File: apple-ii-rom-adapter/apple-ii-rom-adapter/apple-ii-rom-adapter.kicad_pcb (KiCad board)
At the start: 2 copper layers, 51.6 x 43.9 mm, 11 parts, among them J1 ROMSEL, J2 9316 insert, J3 74LS138 insert, U1 28C256, U2 74LS00, U3 74LS138

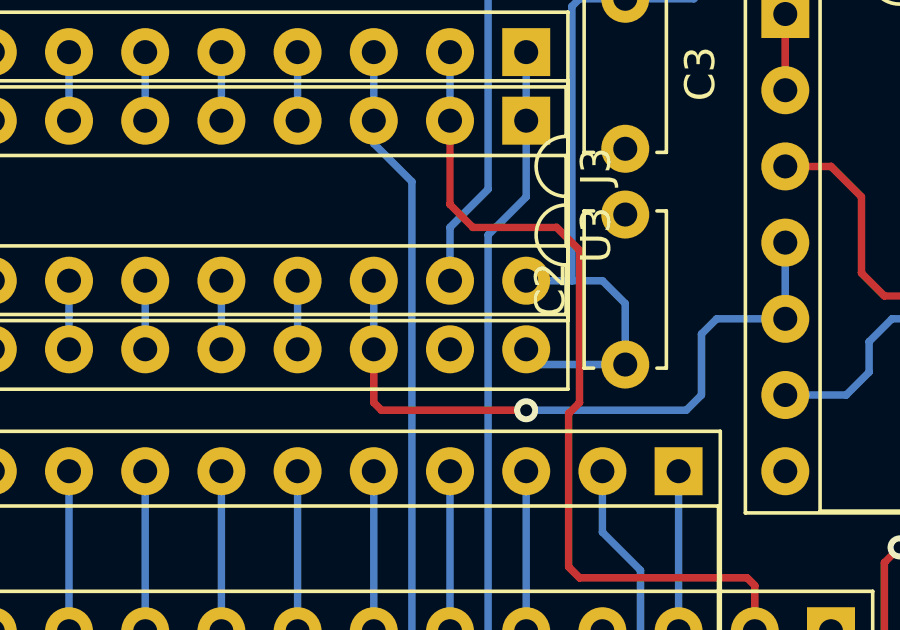
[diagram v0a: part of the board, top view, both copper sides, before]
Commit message: whoops, missed a connection!
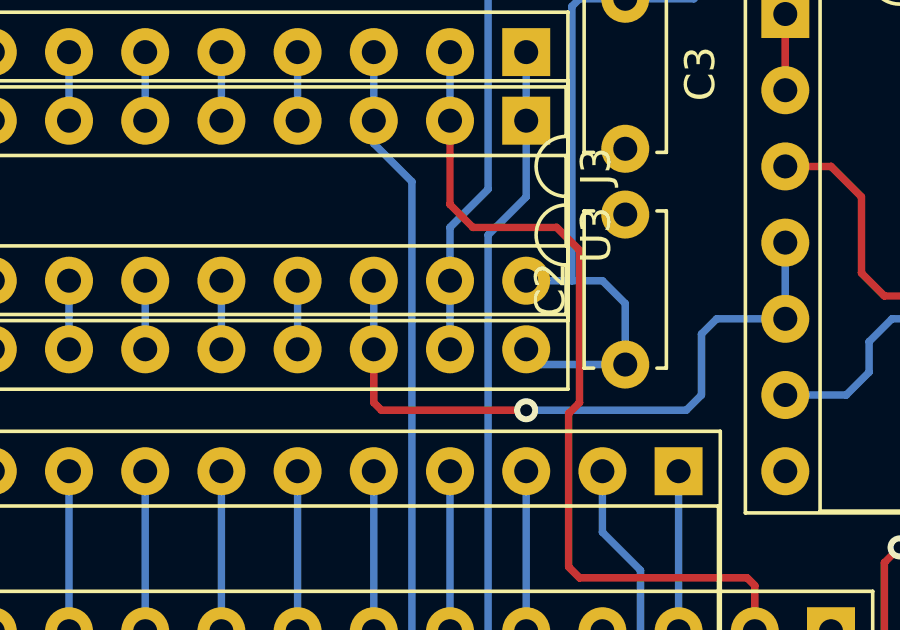
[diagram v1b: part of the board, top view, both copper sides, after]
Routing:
- net A_SEL_0: track 26.0 -> 28.3 mm
